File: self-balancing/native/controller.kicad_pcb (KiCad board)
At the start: 6 copper layers, 38 x 38 mm, 151 parts, among them J101 G, J102 5V, J103 T1, J104 R1, J105 G, J106 5V, J107 T2, J108 R2, J109 G, J110 5V, J111 T3, J112 R3, J113 G, J114 5V, J115 T4, J116 R4, J117 G, J118 3V3, J119 SCL, J120 SDA, J121 INT, J122 G, J123 G, J124 3V3, J125 SCK, J126 MISO, J127 MOSI, J128 CS, J129 G, J130 3V3, J131 CAN_RX, J132 CAN_TX, J133 G, J134 OUT1, J135 OUT2, J136 OUT3, J137 OUT4, J138 G, J139 OUT5, J140 OUT6, J141 OUT7, J142 OUT8, J143 G_LINK, J144 5V_LINK, J145 LINK_TX, J146 LINK_RX, J147 RUN, J148 M_OK, J149 G, J150 VTREF, J151 SWDIO, J152 SWCLK, J153 NRST, J154 BOOT, J155 G, J156 3V3, J157 ADC1, J158 ADC2, J159 ADC3, J160 RPM, J161 G, J162 3V3, J163 LED, J164 BUZ, J165 PC8, J166 PC9, J167 PD14, J2 TYPE-C-31-M-12, J3 MOTOR / 6-wire, J4 EXT SPI SENSOR, J5 GPS / UART4, Q1 2N7002, Q2 DMN2310UW-7, U1 STM32H743VIT6, U10 SN74LVC2G17DBVR, U11 W25N01GVZEIG / 128MiB, U12 TLV803EA29DBZR, U13 TPS2116DRLR, U2 TPS62162DSGR / 3.3V, U3 ICM-42688-P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

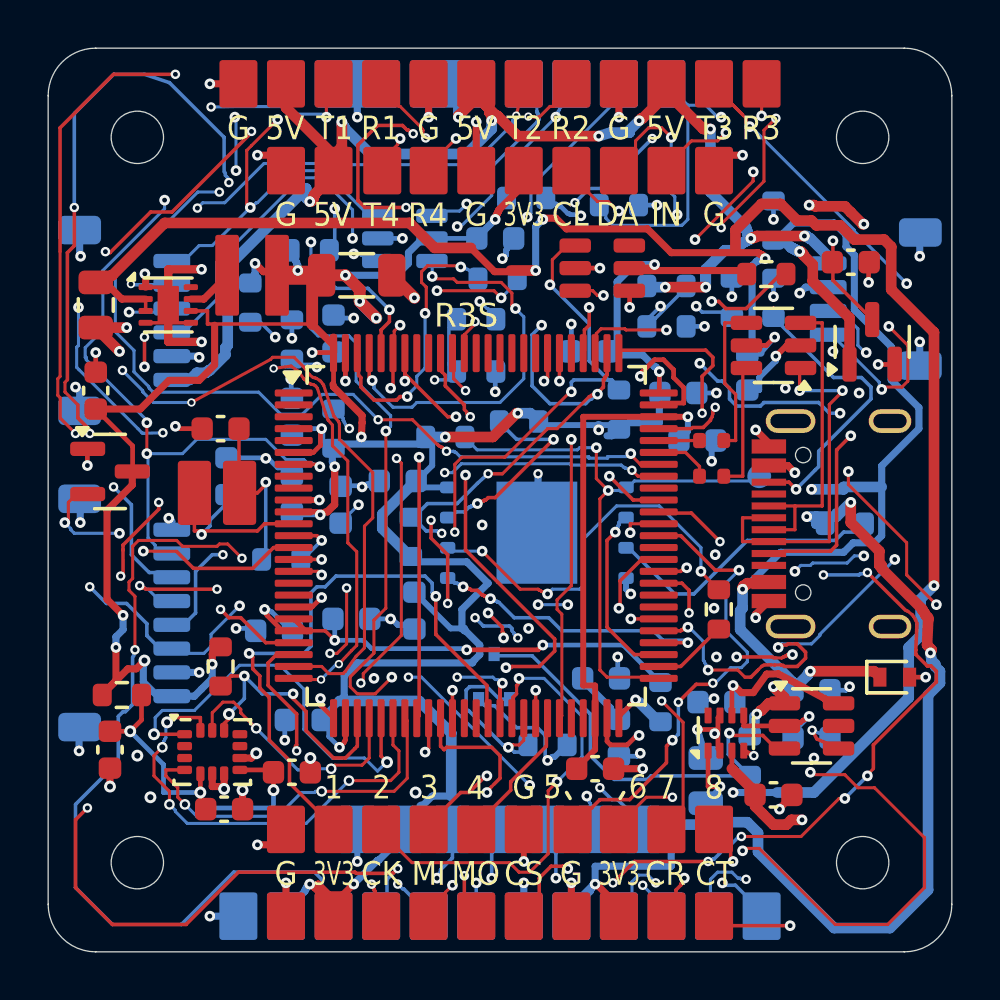
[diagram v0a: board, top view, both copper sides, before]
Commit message: merged small segments
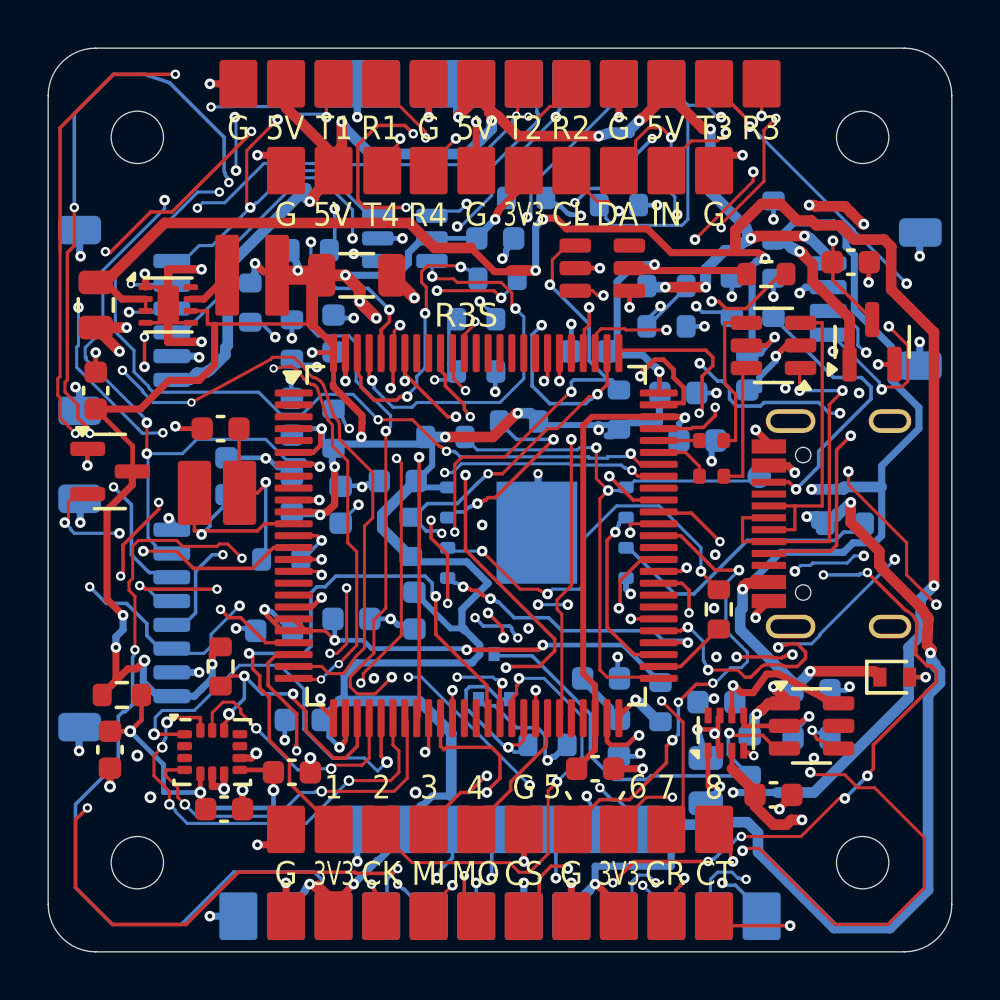
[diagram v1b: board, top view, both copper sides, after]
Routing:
- net SWCLK: track 52.2 -> 54.3 mm
- net VCAP: track 21.2 -> 20.5 mm
